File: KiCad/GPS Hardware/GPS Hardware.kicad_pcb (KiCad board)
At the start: 4 copper layers, 100 x 40 mm, 76 parts, among them J1 USB_C_Receptacle_USB2.0, J2 Conn_01x06_Male, J3 Conn_Coaxial, J4 SIM8051-6-0-14-01-X-REVD, Q1 BC847, U1 ESD122DMX, U10 ublox_SAM-M8Q, U3 BQ24295, U4 LM3480-3.3, U5 ATmega328-AU, U6 SN74AVC4T774PW, U7 74AVC2T245GU-Q100X, U8 SARA-U201, U9 NCP662SQ33T1G, Y1 Crystal

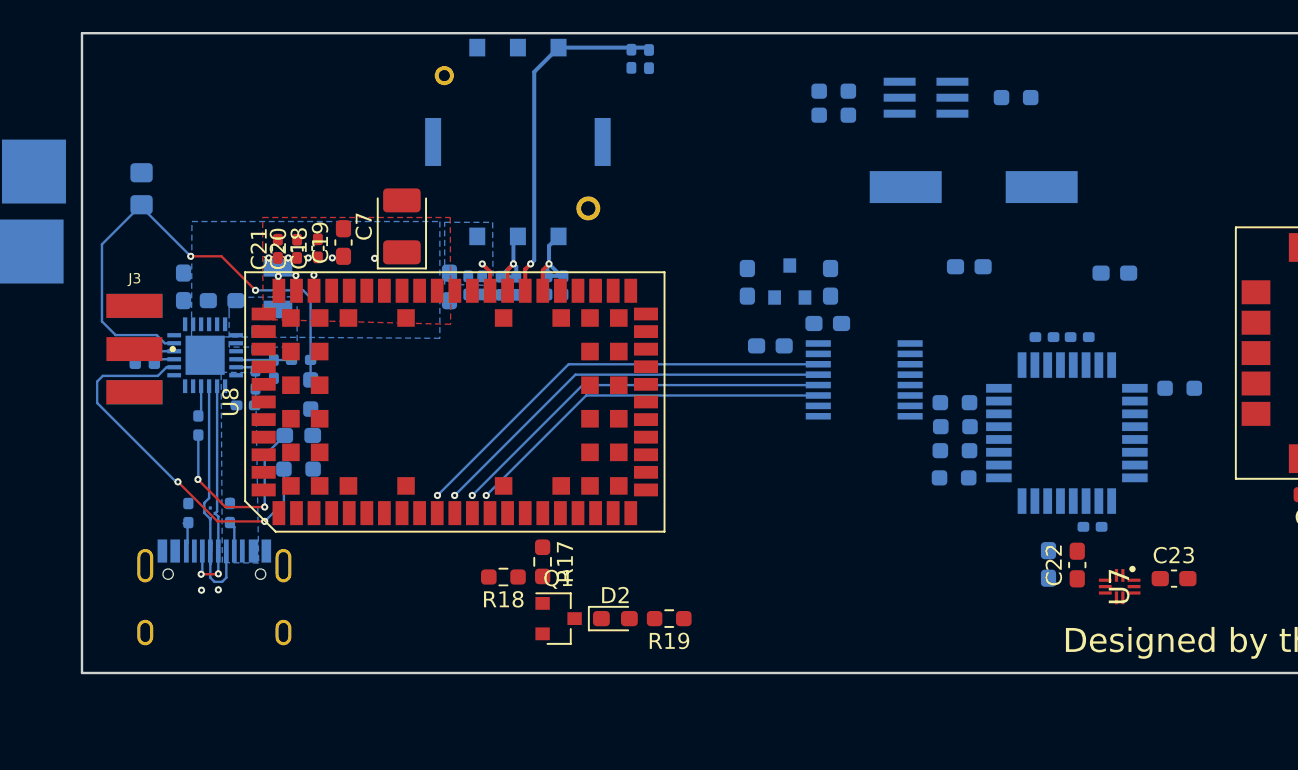
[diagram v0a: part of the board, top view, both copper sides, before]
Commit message: Update (again :+1:  )
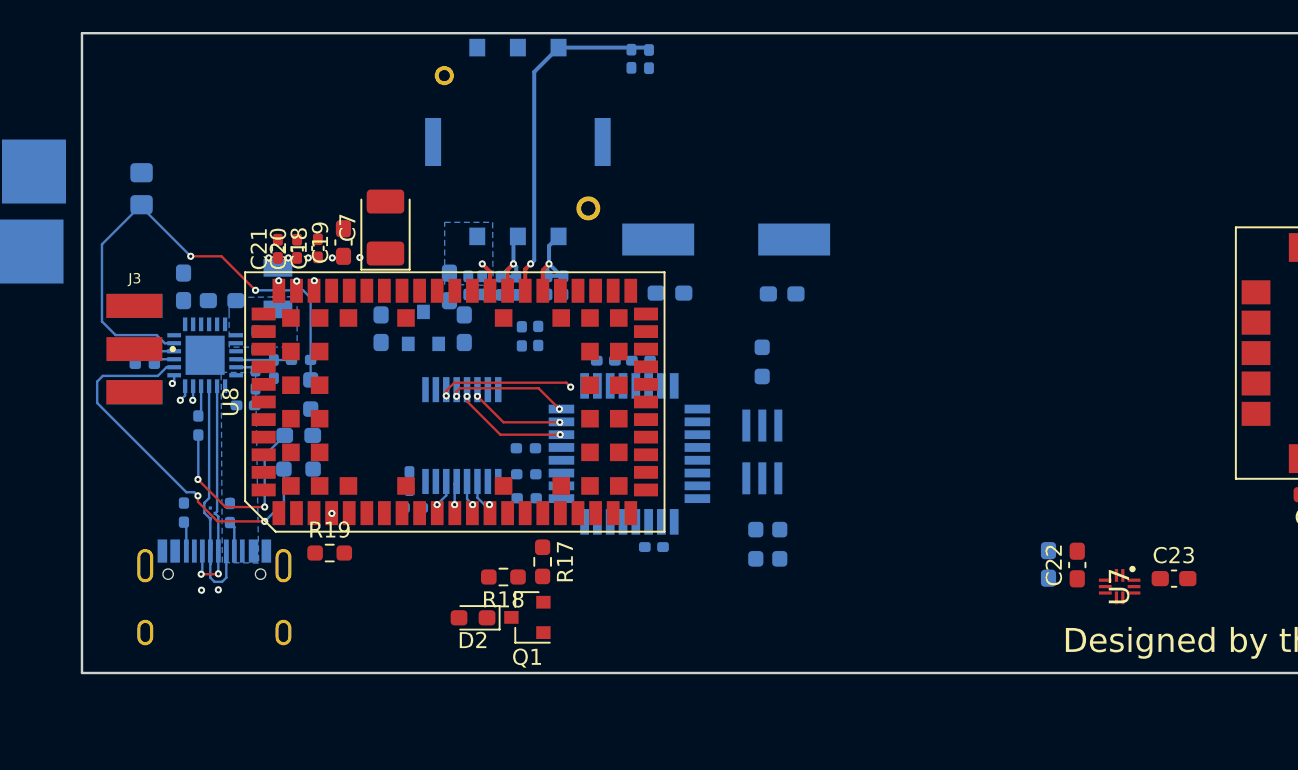
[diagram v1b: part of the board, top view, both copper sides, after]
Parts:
- C16, C17: footprint Capacitor_SMD:C_0603_1608Metric_Pad1.08x0.95mm_HandSolder -> Capacitor_SMD:C_0402_1005Metric_Pad0.74x0.62mm_HandSolder
- R15, R16, R3, R4, R5: footprint Resistor_SMD:R_0603_1608Metric_Pad0.98x0.95mm_HandSolder -> Resistor_SMD:R_0402_1005Metric_Pad0.72x0.64mm_HandSolder
- moved R5 40.2 mm to (128.5, 78.9), turned to 90 degrees
- moved R14 28.7 mm to (142.1, 92.0), turned to 270 degrees
- moved C17 27.9 mm to (120.5, 88.0), turned to 270 degrees
- moved R3 27.7 mm to (127.5, 79.0), turned to 90 degrees
- moved C12 27.5 mm to (134.9, 80.5)
- moved C13 27.5 mm to (132.8, 80.5)
- moved C11 27.4 mm to (135.8, 92.1)
- moved U5 27.4 mm to (134.2, 86.3)
- moved R13 27.0 mm to (143.6, 92.0), turned to 270 degrees
- moved R15 27.0 mm to (127.8, 86.0)
- moved R4 26.8 mm to (127.8, 87.6)
- moved R16 26.8 mm to (127.8, 89.1)
- moved U6 25.4 mm to (123.8, 85.2), turned to 270 degrees
- moved C16 24.5 mm to (120.7, 89.7)
- moved J2 24.4 mm to (142.5, 86.2), turned to 90 degrees
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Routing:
- net RTS_Cellular: track 27.2 -> 1.69 mm
- net CTS_Cellular: track 25.9 -> 1.50 mm
- net TX_Cellular: track 24.5 -> 1.59 mm
- net RX_Cellular: track 23.3 -> 1.95 mm
- net CTS: track 0.00 -> 8.42 mm, vias 0 -> 2
- net RTS: track 0.00 -> 7.36 mm, vias 0 -> 2
- net RX: track 0.00 -> 7.01 mm, vias 0 -> 2
- net TX: track 0.00 -> 5.82 mm, vias 0 -> 2
- net SDA_Power: track 0.00 -> 1.00 mm, vias 0 -> 1
- net SCL_Power: track 0.00 -> 0.89 mm, vias 0 -> 1
- net Net-(J1-PadB5): track 1.83 -> 2.40 mm
- net INT_Power: track 0.00 -> 0.56 mm, vias 0 -> 1
- net +1V8: vias 0 -> 1
- removed copper zone on B.Cu, net SYS
- removed copper zone on F.Cu, net SYS
